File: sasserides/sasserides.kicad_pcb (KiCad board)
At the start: 2 copper layers, 170 x 80 mm, 134 parts, among them J1 Conn_02x16_Odd_Even, Q1 2N7002, U1 CDCV304PW

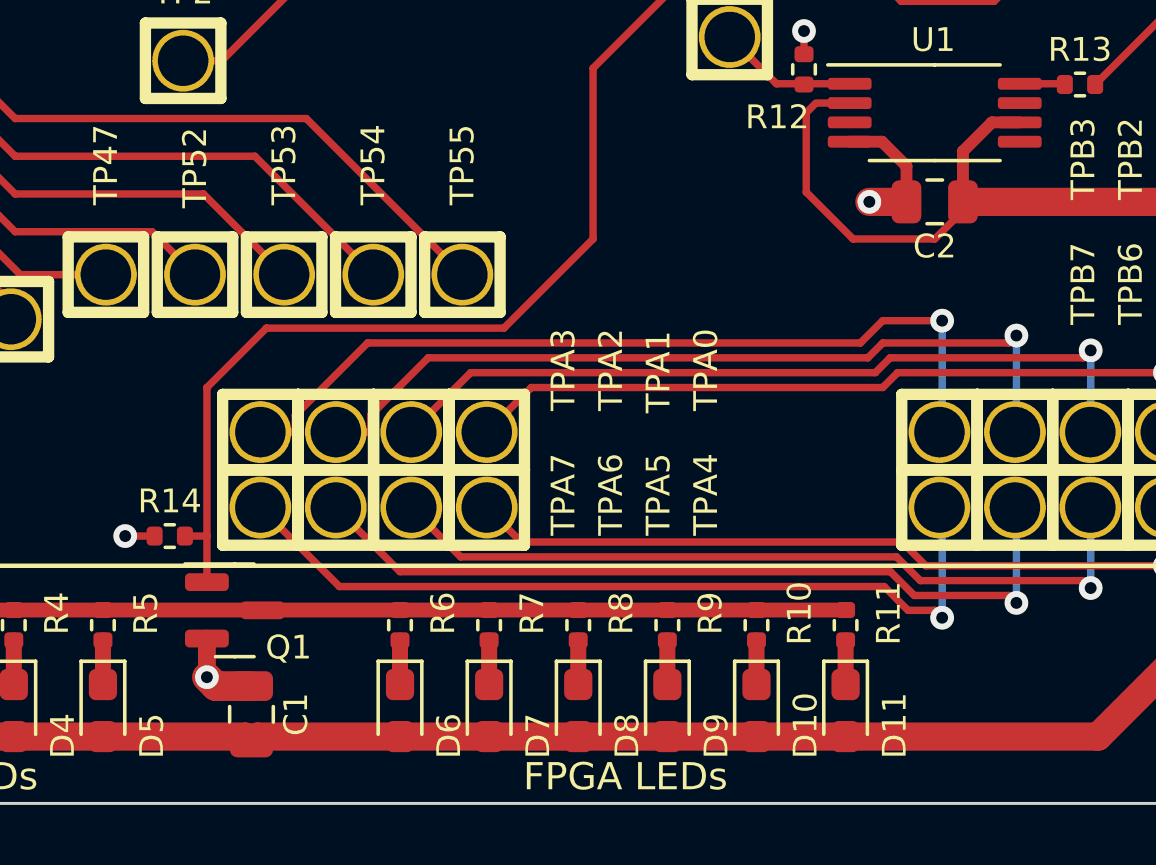
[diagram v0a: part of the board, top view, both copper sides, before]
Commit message: Update Sasserides PCB
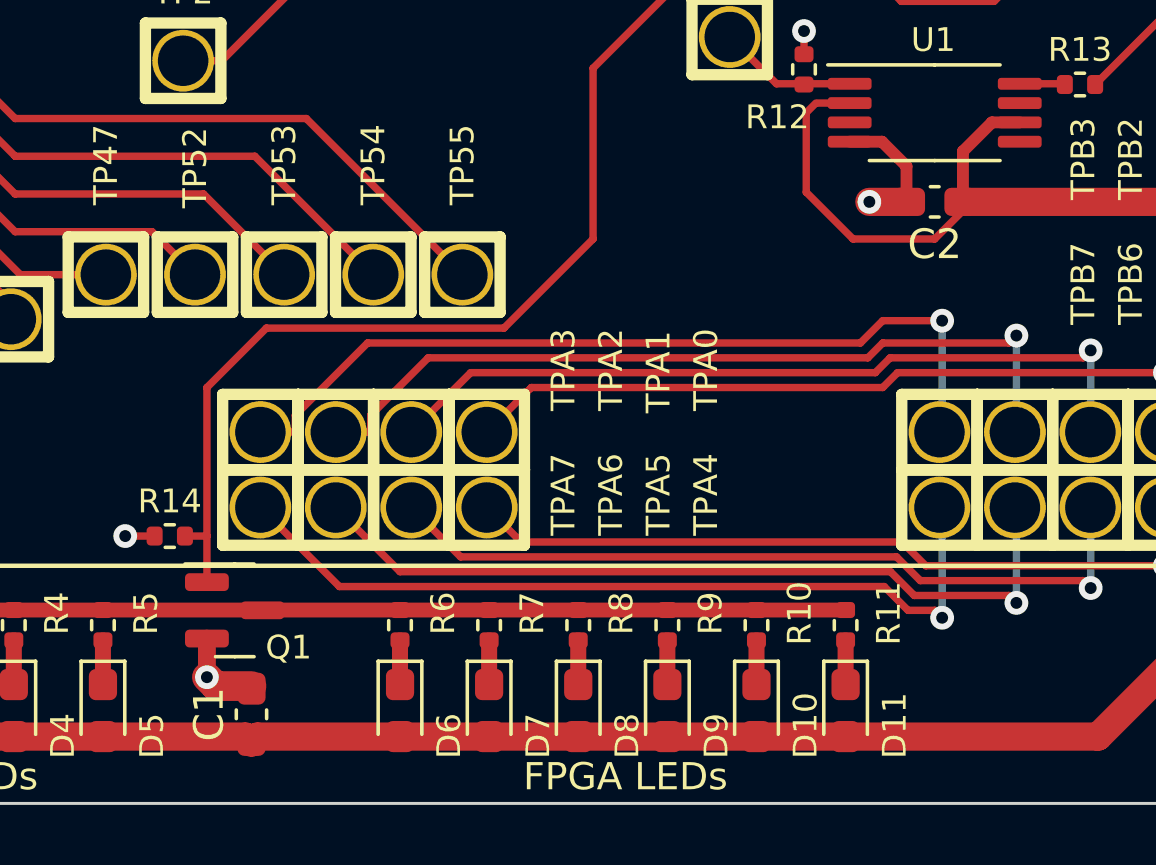
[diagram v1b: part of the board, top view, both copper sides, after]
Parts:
- C1, C2: footprint Capacitor_SMD:C_0805_2012Metric -> Capacitor_SMD:C_0603_1608Metric_Pad1.08x0.95mm_HandSolder
